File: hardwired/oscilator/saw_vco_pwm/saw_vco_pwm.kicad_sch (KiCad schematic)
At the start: 26 parts, among them Q1 NPN, Q2 PNP, Q4 NPN, Q5 PNP, U1 ${SIM.PARAMS}, U2 ${SIM.PARAMS}, U3 ${SIM.PARAMS}, U4 ${SIM.PARAMS}, U5 ${SIM.PARAMS}

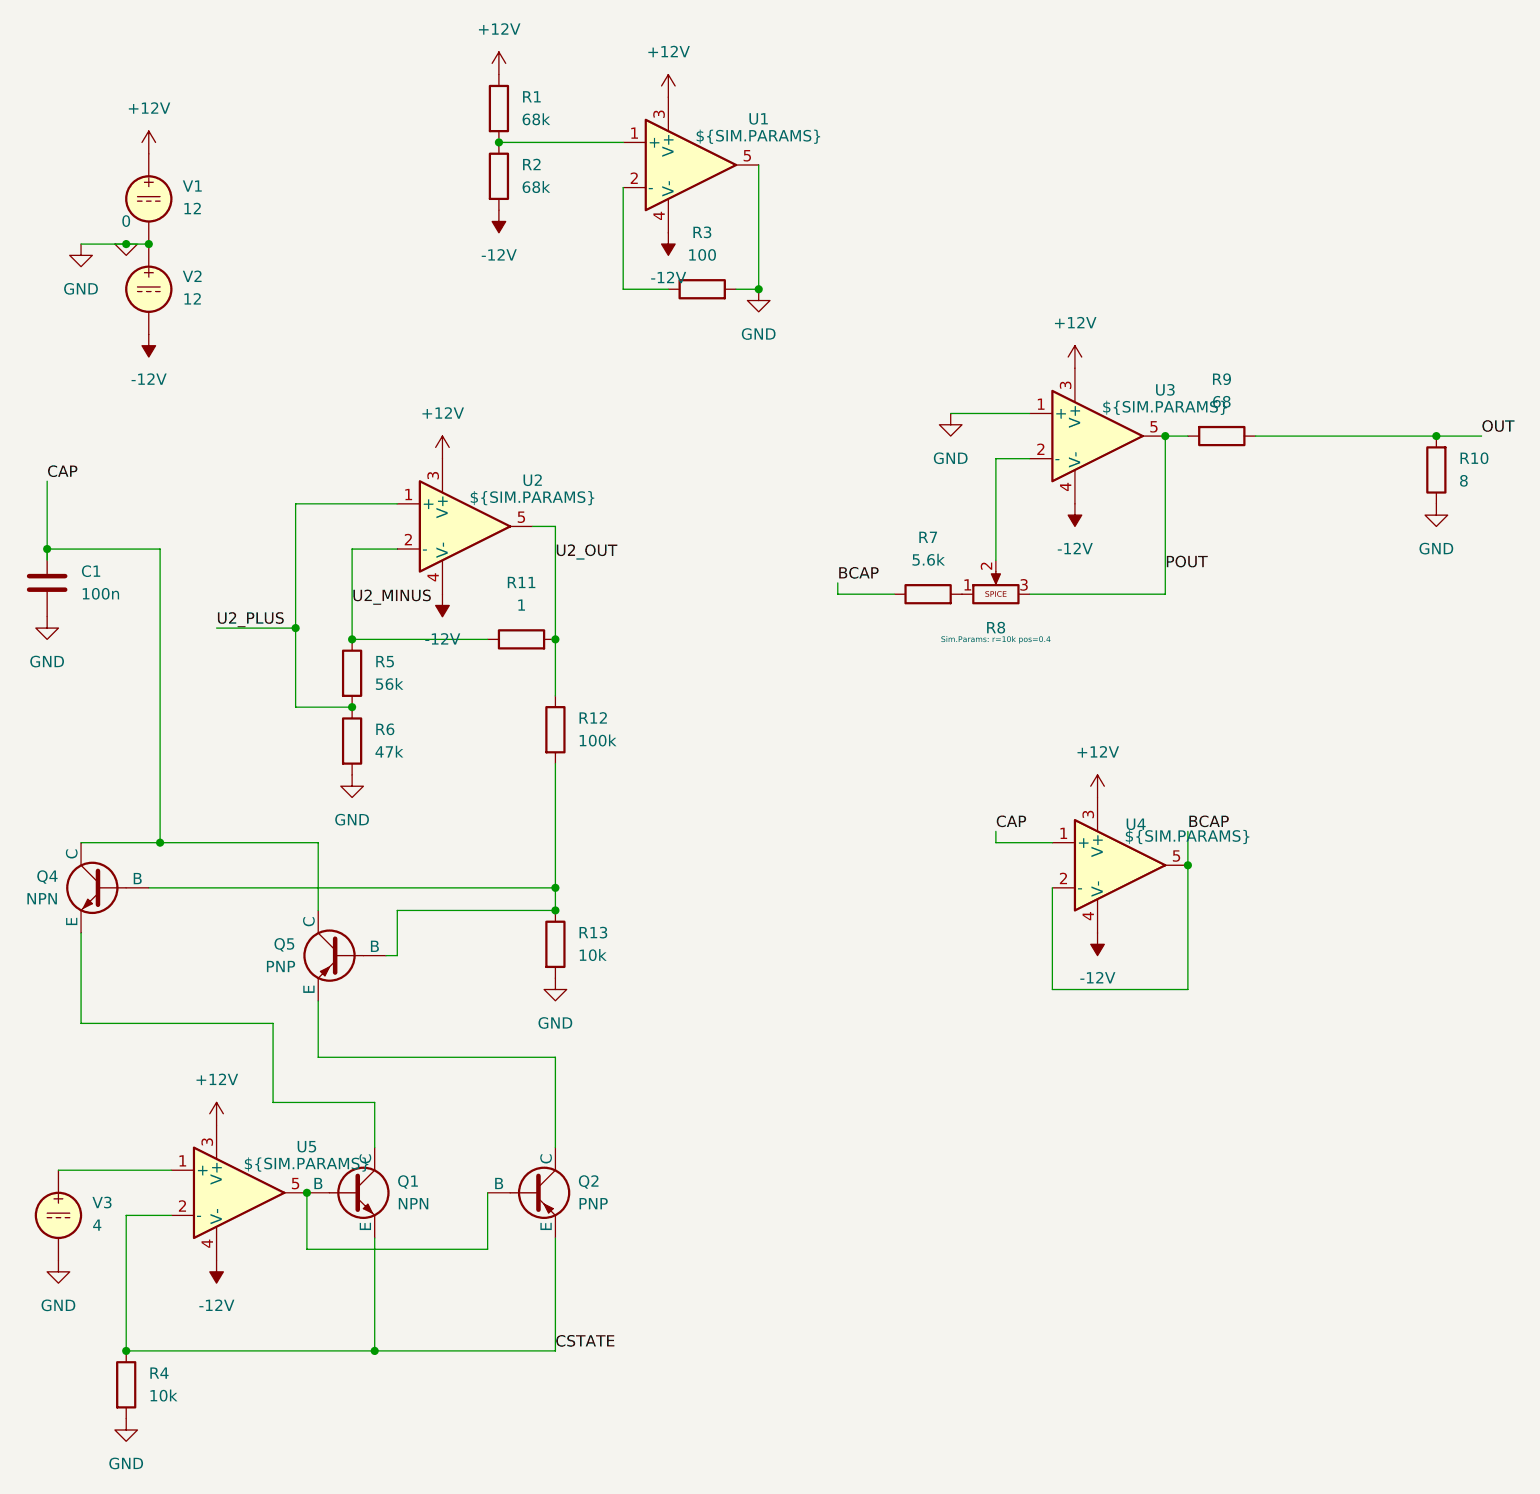
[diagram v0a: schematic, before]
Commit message: Many Kicad drawings
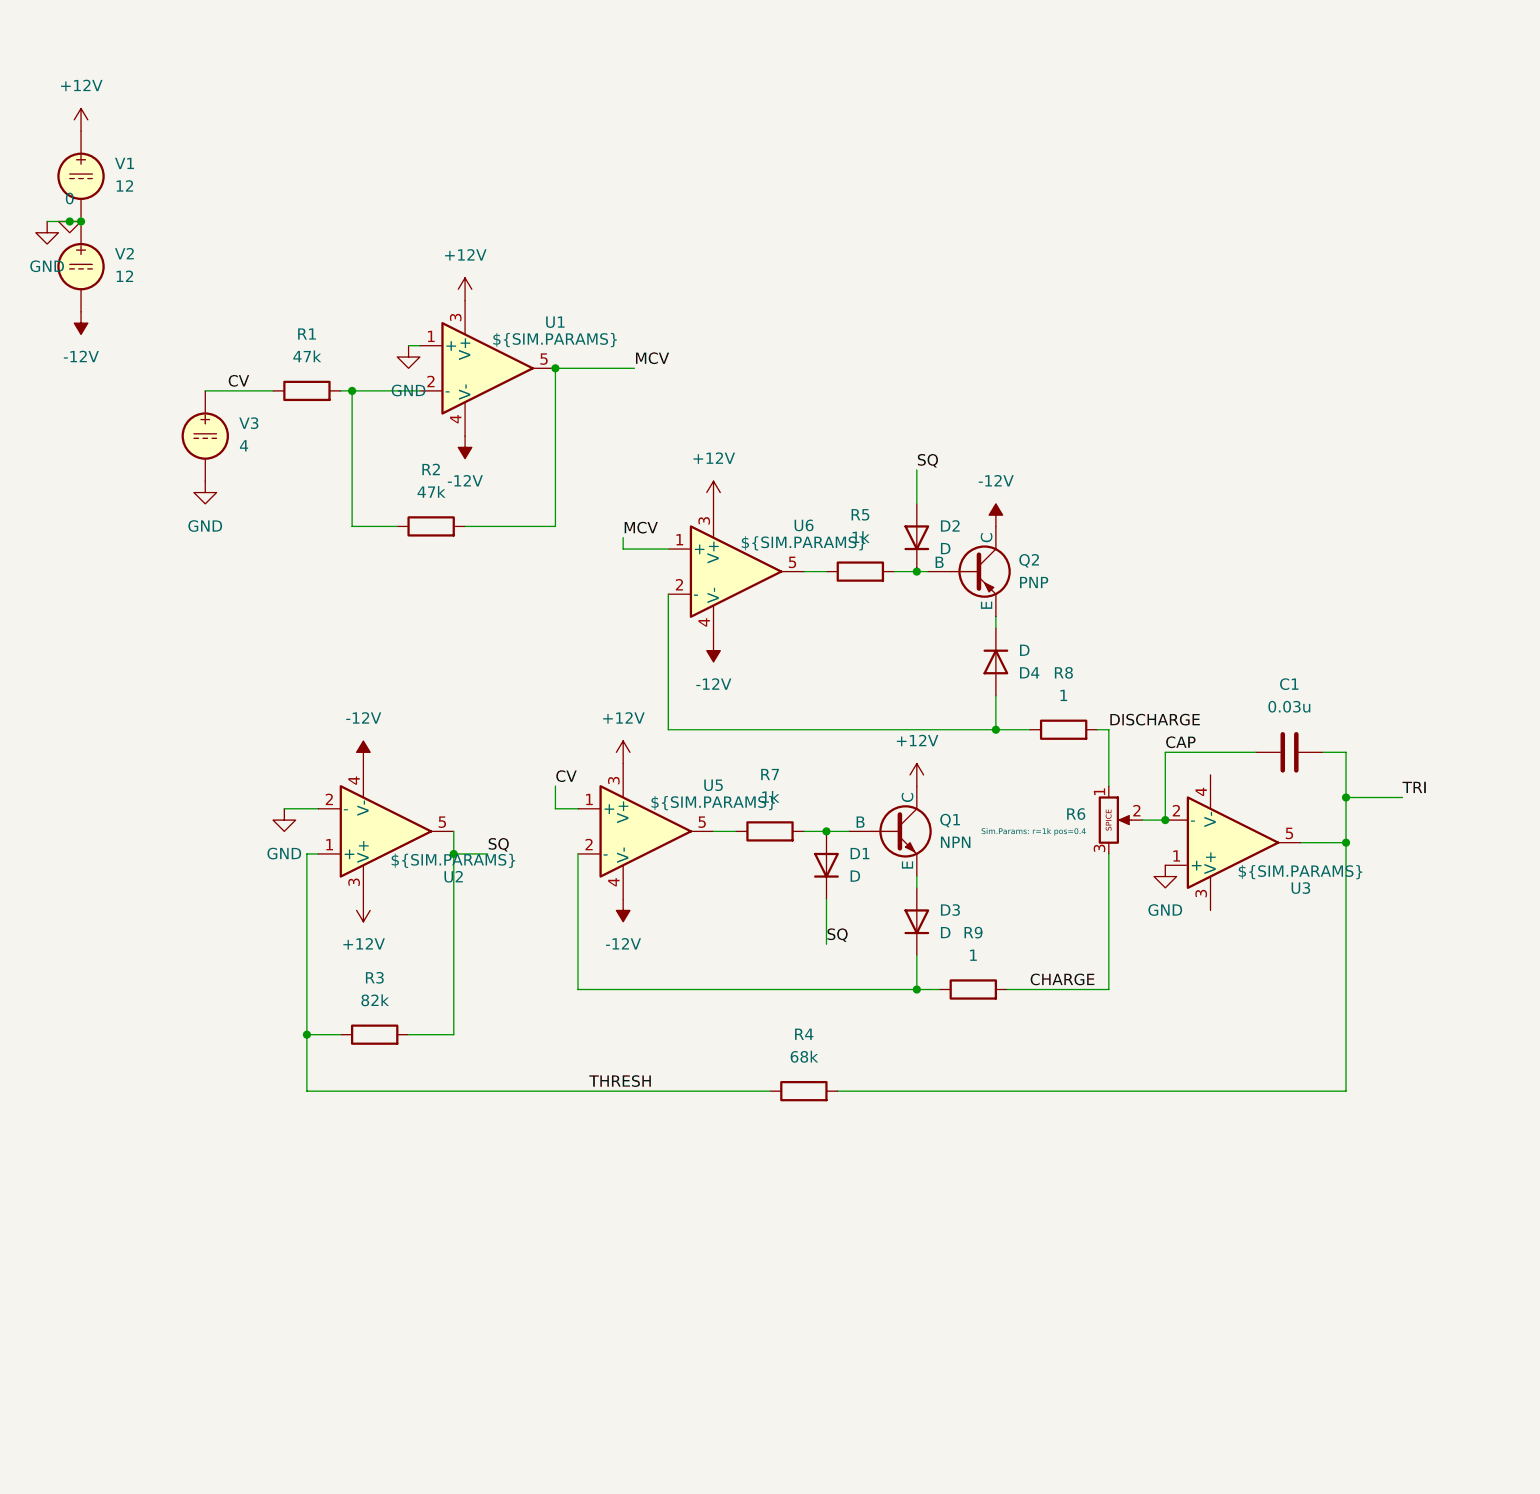
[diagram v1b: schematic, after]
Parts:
- removed Q4: NPN, symbol Simulation_SPICE:NPN
- removed Q5: PNP, symbol Simulation_SPICE:PNP
- removed R10: 8, symbol Device:R
- removed R11: 1, symbol Device:R
- removed R12: 100k, symbol Device:R
- removed R13: 10k, symbol Device:R
- removed R6: 47k, symbol Device:R
- removed R8: Potentiometer, symbol Simulation_SPICE:Potentiometer
- removed U4: ${SIM.PARAMS}, symbol Simulation_SPICE:OPAMP
- added D1, D2, D3, D4: D, symbol Device:D
- added R6: Potentiometer, symbol Simulation_SPICE:Potentiometer
- added R8: 1, symbol Device:R
- added U6: ${SIM.PARAMS}, symbol Simulation_SPICE:OPAMP
- C1: value 100n -> 0.03u
- R1, R2: value 68k -> 47k
- R3: value 100 -> 82k
- R4: value 10k -> 68k
- R5: value 56k -> 1k
- R7: value 5.6k -> 1k
- R9: value 68 -> 1
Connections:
- net +12V: now also Q1.1 (C), U6.3 (V+); no longer R1.1, U3.3 (V+)
- net -12V: now also Q2.1 (C), U6.4 (V-); no longer R2.2, U3.4 (V-)
- net 0: now also U1.1 (+), U2.2 (-); no longer C1.2, R3.2, R4.2, U1.5
- net CAP: now also U3.2 (-), R6.2
- net CV: now reaches U5.1 (+), V3.1
- net CV: now also R1.1
- net at U1.2 (-): now also R1.2, R2.1; no longer R3.1
- net at R7.2: now also Q1.2 (B), D1.2 (A)
- net BCAP: no longer names the net of R7.1
- net BCAP: now also U5.5
- removed net CSTATE: Q1.3 (E), Q2.3 (E), R4.1, U5.2 (-)
- net OUT: no longer names the net of R9.1
- net OUT: now also U5.2 (-), D3.1 (K)
- net POUT renamed CHARGE
- net CHARGE: now also R6.3; no longer U3.5
- net U2_MINUS: no longer names the net of R5.1
- net U2_MINUS: now also U6.5; no longer U2.2 (-)
- net U2_OUT renamed SQ
- net SQ: now also R3.2, D1.1 (K), D2.2 (A)
- net U2_PLUS: no longer names the net of R5.2
- net U2_PLUS: now also Q2.2 (B), D2.1 (K); no longer U2.1 (+)
- new net: D4.1 (K), Q2.3 (E)
- new net: D4.2 (A), R8.1, U6.2 (-)
- new net: D3.2 (A), Q1.3 (E)
- new net DISCHARGE: R6.1, R8.2
- new net MCV: R2.2, U1.5, U6.1 (+)
- new net THRESH: R3.1, R4.1, U2.1 (+)
- new net TRI: C1.2, R4.2, U3.5
